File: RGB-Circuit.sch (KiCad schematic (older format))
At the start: 168 parts

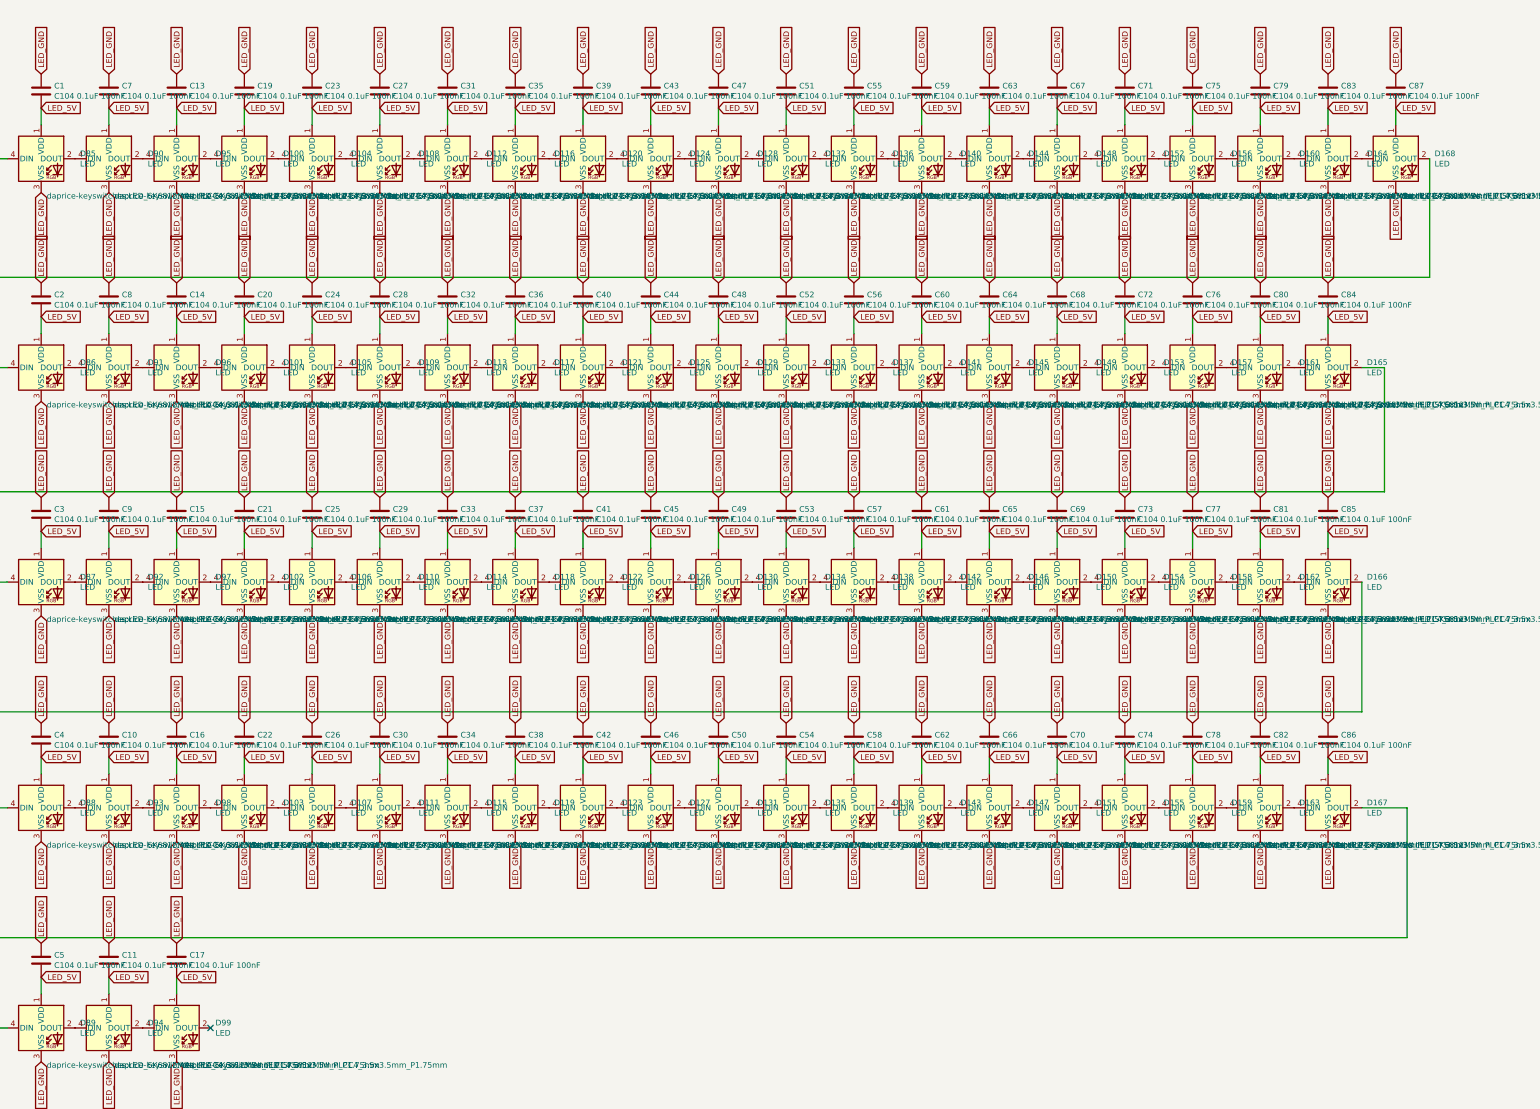
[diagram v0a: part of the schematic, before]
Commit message: working on the chip
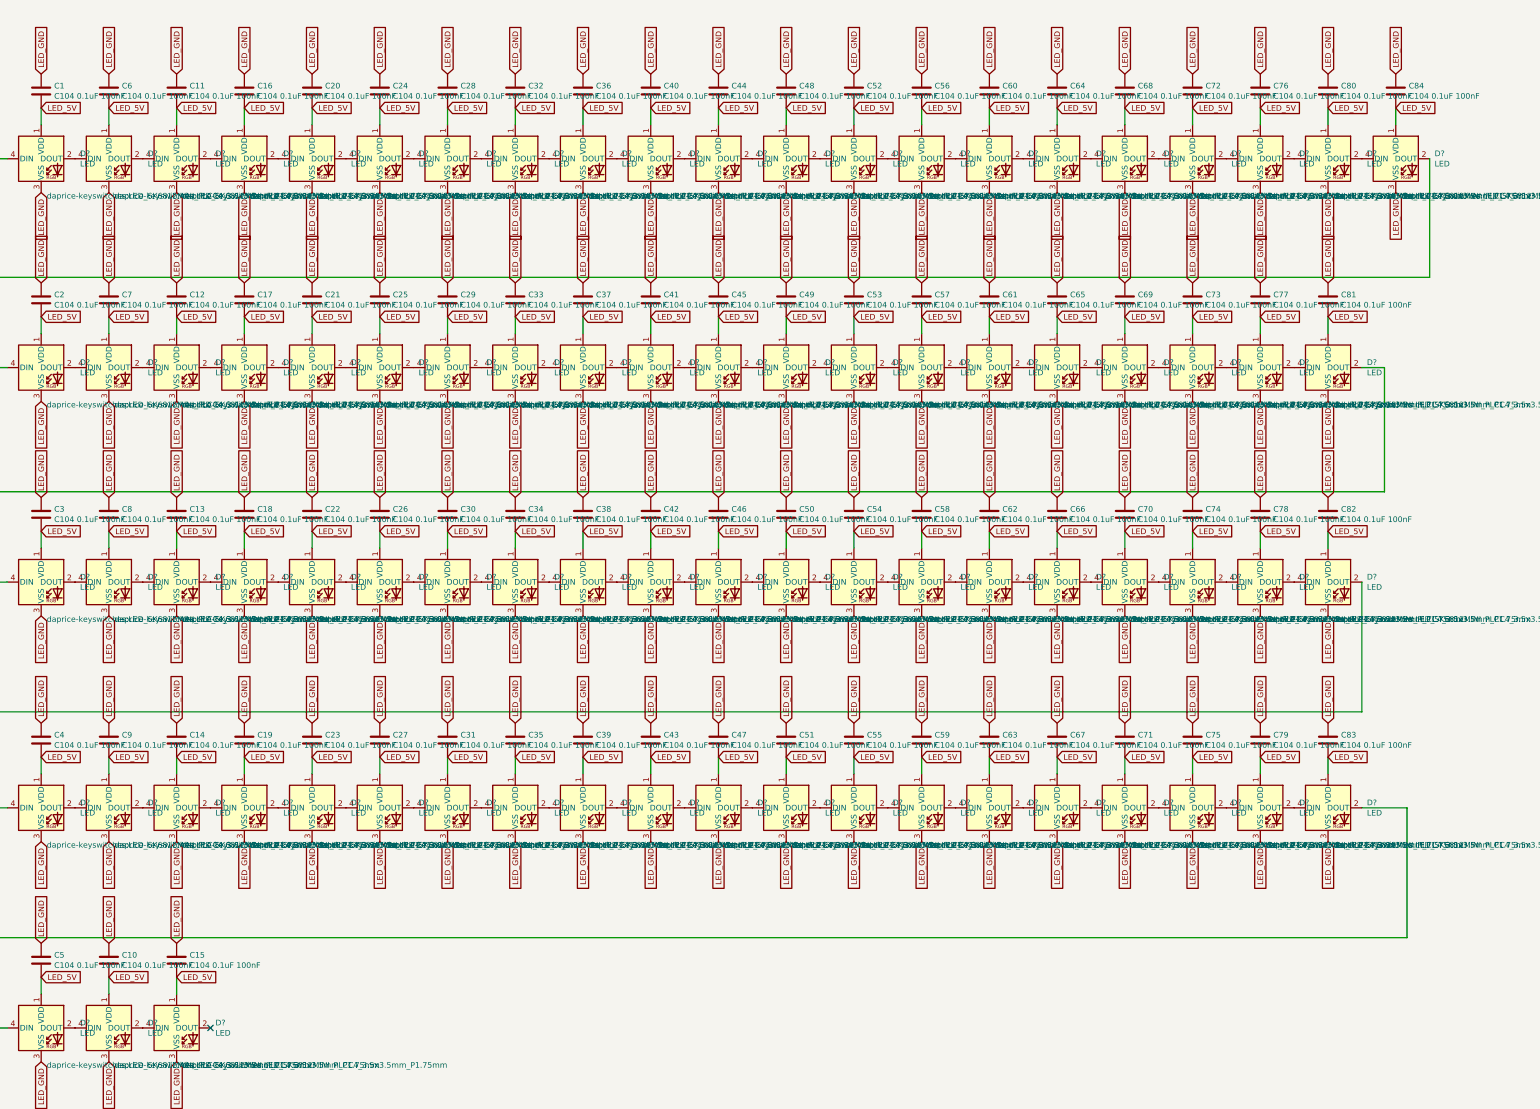
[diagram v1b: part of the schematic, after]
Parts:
- renumbered C11 to C10, C13 to C11, C14 to C12, C15 to C13, C16 to C14, C17 to C15, C19 to C16, C20 to C17, C21 to C18, C22 to C19, C23 to C20, C24 to C21, C25 to C22, C26 to C23, C27 to C24, C28 to C25, C29 to C26, C30 to C27, C31 to C28, C32 to C29, C33 to C30, C34 to C31, C35 to C32, C36 to C33, C37 to C34, C38 to C35, C39 to C36, C40 to C37, C41 to C38, C42 to C39, C43 to C40, C44 to C41, C45 to C42, C46 to C43, C47 to C44, C48 to C45, C49 to C46, C50 to C47, C51 to C48, C52 to C49, C53 to C50, C54 to C51, C55 to C52, C56 to C53, C57 to C54, C58 to C55, C59 to C56, C60 to C57, C61 to C58, C62 to C59, C7 to C6, C63 to C60, C64 to C61, C65 to C62, C66 to C63, C67 to C64, C68 to C65, C69 to C66, C70 to C67, C71 to C68, C72 to C69, C8 to C7, C73 to C70, C74 to C71, C75 to C72, C76 to C73, C77 to C74, C78 to C75, C79 to C76, C80 to C77, C81 to C78, C82 to C79, C9 to C8, C83 to C80, C84 to C81, C85 to C82, C86 to C83, C87 to C84, C10 to C9, D85 to D?, D90 to D?, D95 to D?, D100 to D?, D104 to D?, D108 to D?, D112 to D?, D116 to D?, D120 to D?, D124 to D?, D128 to D?, D132 to D?, D136 to D?, D140 to D?, D144 to D?, D148 to D?, D152 to D?, D156 to D?, D160 to D?, D164 to D?, D168 to D?, D86 to D?, D91 to D?, D96 to D?, D101 to D?, D105 to D?, D109 to D?, D113 to D?, D117 to D?, D121 to D?, D125 to D?, D129 to D?, D133 to D?, D137 to D?, D141 to D?, D145 to D?, D149 to D?, D153 to D?, D157 to D?, D161 to D?, D165 to D?, D87 to D?, D92 to D?, D97 to D?, D102 to D?, D106 to D?, D110 to D?, D114 to D?, D118 to D?, D122 to D?, D126 to D?, D130 to D?, D134 to D?, D138 to D?, D142 to D?, D146 to D?, D150 to D?, D154 to D?, D158 to D?, D162 to D?, D166 to D?, D88 to D?, D93 to D?, D98 to D?, D103 to D?, D107 to D?, D111 to D?, D115 to D?, D119 to D?, D123 to D?, D127 to D?, D131 to D?, D135 to D?, D139 to D?, D143 to D?, D147 to D?, D151 to D?, D155 to D?, D159 to D?, D163 to D?, D167 to D?, D89 to D?, D94 to D?, D99 to D?

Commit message: RGB circuit rescue cleanup
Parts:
- D? (x84): symbol chgray-keyboard-rescue:SK6812MINI-Cherry-Symbol -> LED:SK6812MINI

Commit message: update keyboard
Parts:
- gave numbers to parts that had none: 84
